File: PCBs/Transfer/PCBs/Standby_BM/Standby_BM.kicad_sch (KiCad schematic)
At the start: 30 parts, among them J1 SARI, J10 BL OUT, J11 5V IN, J12 LCD OUT 5V, J16 Address Select 0, J17 Address Select 1, J18 VVI PWR, J19 STBY AIR, J2 LOWER PWR, J20 AIR STPR, J21 AIR PWR, J3 UPPER PWR, J4 RWR BRT (ANALOG), J5 OLED PWR SEL, J6 STANDBY ALT, J7 STBY VVI, J8 VVI STPR, J9 BL IN, P1 Power, P2 Analog, P3 Analog, P4 Digital, P5 PWM, P6 PWM, P7 Communication

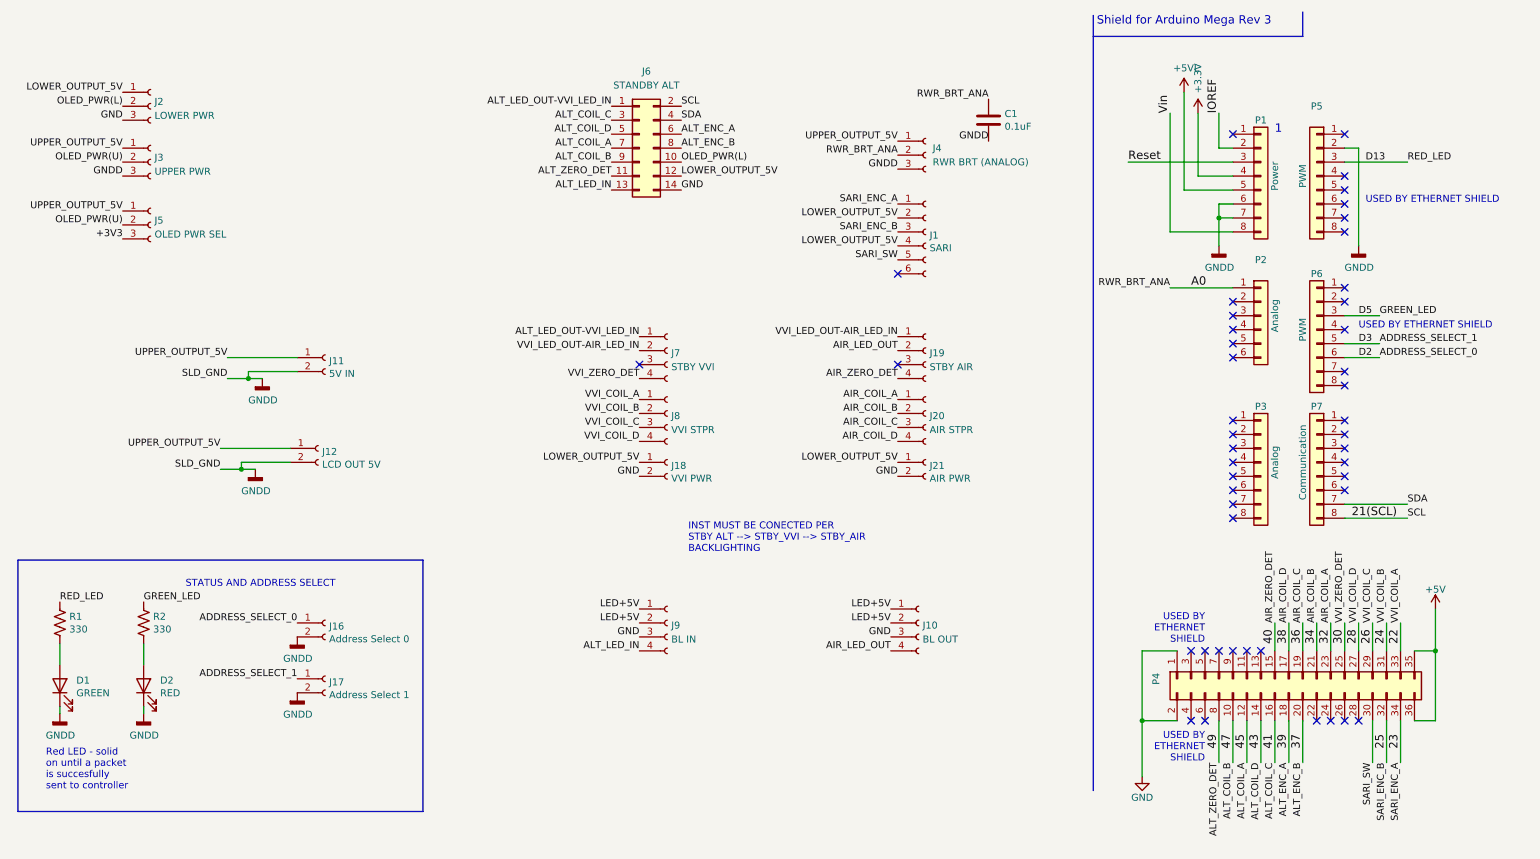
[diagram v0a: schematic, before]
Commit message: Ben4
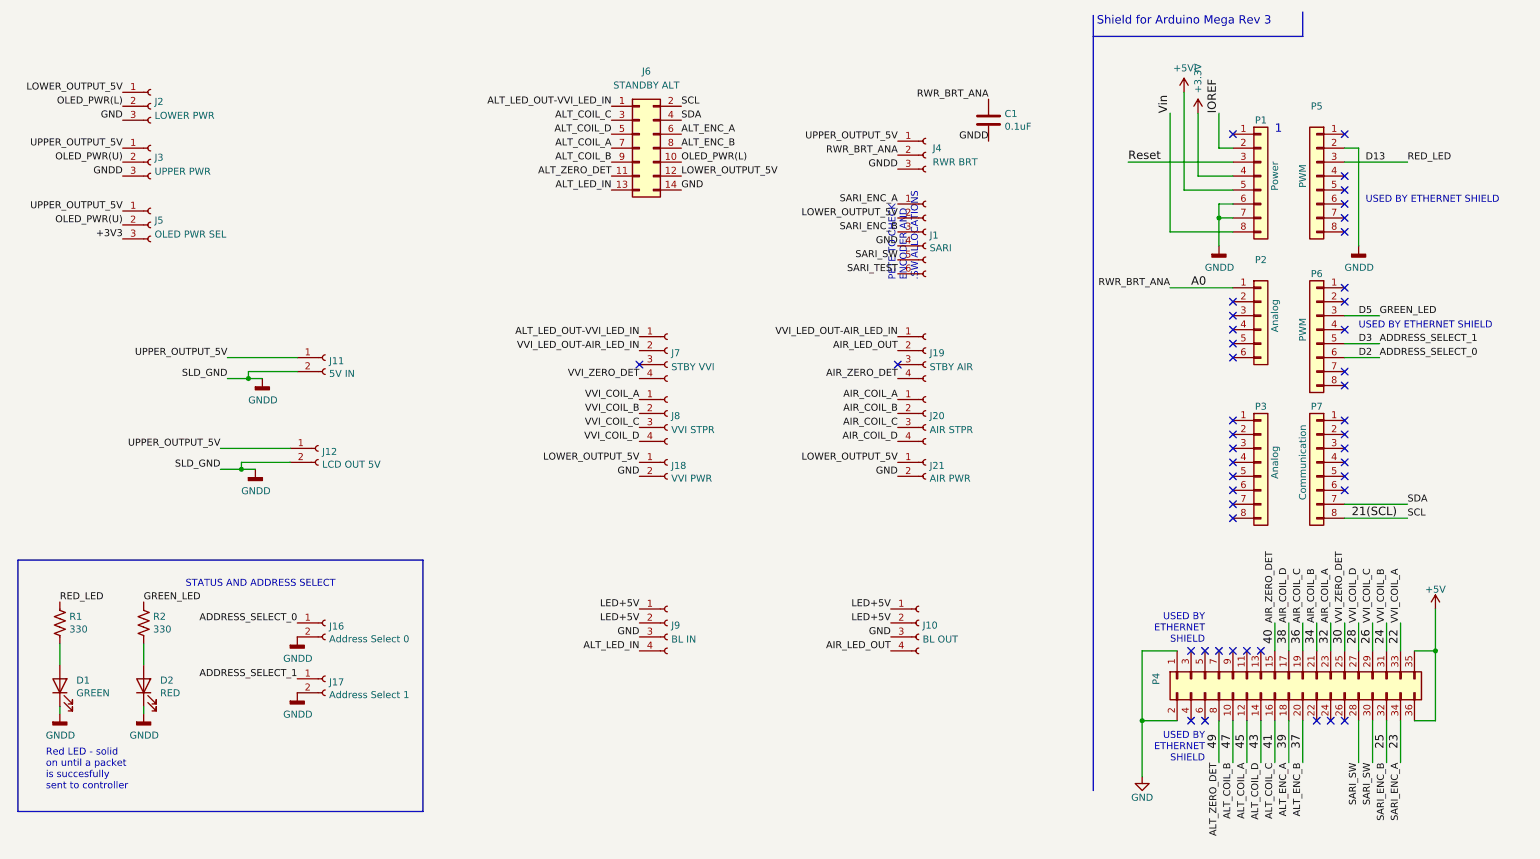
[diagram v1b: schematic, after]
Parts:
- J18, J21: footprint Connector_Molex:Molex_KK-254_AE-6410-06A_1x02_P2.54mm_Vertical -> Connector_Molex:Molex_KK-254_AE-6410-02A_1x02_P2.54mm_Vertical
- J2, J3: footprint Connector_Molex:Molex_KK-254_AE-6410-06A_1x03_P2.54mm_Vertical -> Connector_Molex:Molex_KK-254_AE-6410-03A_1x03_P2.54mm_Vertical
- J20, J7, J8: footprint Connector_Molex:Molex_KK-254_AE-6410-06A_1x04_P2.54mm_Vertical -> Connector_Molex:Molex_KK-254_AE-6410-04A_1x04_P2.54mm_Vertical
- J4: value RWR BRT (ANALOG) -> RWR BRT; footprint Connector_Molex:Molex_KK-254_AE-6410-06A_1x03_P2.54mm_Vertical -> Connector_Molex:Molex_KK-254_AE-6410-03A_1x03_P2.54mm_Vertical
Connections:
- net GND: now also J1.4 (Pin_4)
- net LOWER_OUTPUT_5V: no longer J1.4 (Pin_4)
- net SARI_SW: now also P4.28 (Pin_28)
- net SARI_TEST: now reaches J1.6 (Pin_6)
- no-connect marks 46 -> 44
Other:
- note added: "PETE TO CHECK ENCODER AND .SW ALLOCATIONS"
- note removed: "INST MUST BE CONECTED PER STBY ALT --> STBY_VVI --> STBY_AIR BACKLIGHTING"
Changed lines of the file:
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@@
   (no_connect (at 234.95 128.27))
   (no_connect (at 257.81 49.53))
-  (no_connect (at 176.53 59.69))
   (no_connect (at 242.57 128.27))
   (no_connect (at 257.81 41.91))
@@
   (no_connect (at 257.81 80.01))
   (no_connect (at 257.81 93.98))
-  (no_connect (at 260.35 140.97))
   (no_connect (at 237.49 67.31))
   (no_connect (at 257.81 88.9))
@@
     (stroke (width 0) (type default) (color 0 0 0 0))
   )
+  (wire (pts (xy 260.35 140.97) (xy 260.35 148.59))
+    (stroke (width 0) (type default) (color 0 0 0 0))
+  )
   (wire (pts (xy 54.61 74.93) (xy 67.31 74.93))
     (stroke (width 0) (type default) (color 0 0 0 0))
@@
     (effects (font (size 1.524 1.524)) (justify left bottom))
   )
-  (text "INST MUST BE CONECTED PER\nSTBY ALT --> STBY_VVI --> STBY_AIR\nBACKLIGHTING"
-    (at 138.43 110.49 0)
+  (text "PETE TO CHECK \nENCODER AND \n.SW ALLOCATIONS" (at 180.34 60.96 90)
     (effects (font (size 1.27 1.27)) (justify left bottom))
   )
@@
     (effects (font (size 1.27 1.27)) (justify right bottom))
   )
+  (label "SARI_SW" (at 260.35 148.59 270)
+    (effects (font (size 1.27 1.27)) (justify right bottom))
+  )
   (label "UPPER_OUTPUT_5V" (at 35.56 48.26 180)
     (effects (font (size 1.27 1.27)) (justify right bottom))
@@
     (effects (font (size 1.27 1.27)) (justify right bottom))
   )
+  (label "SARI_TEST" (at 176.53 59.69 180)
+    (effects (font (size 1.27 1.27)) (justify right bottom))
+  )
   (label "VVI_COIL_C" (at 262.89 123.19 90)
     (effects (font (size 1.27 1.27)) (justify left bottom))
   )
-  (label "LOWER_OUTPUT_5V" (at 176.53 54.61 180)
+  (label "GND" (at 176.53 54.61 180)
     (effects (font (size 1.27 1.27)) (justify right bottom))
   )
@@
       (effects (font (size 1.27 1.27)) (justify left))
     )
-    (property "Footprint" "Connector_Molex:Molex_KK-254_AE-6410-06A_1x02_P2.54mm_Vertical" (id 2) (at 181.61 93.98 0)
+    (property "Footprint" "Connector_Molex:Molex_KK-254_AE-6410-02A_1x02_P2.54mm_Vertical" (id 2) (at 181.61 93.98 0)
       (effects (font (size 1.27 1.27)) hide)
     )
@@
       (effects (font (size 1.27 1.27)) (justify left))
     )
-    (property "Footprint" "Connector_Molex:Molex_KK-254_AE-6410-06A_1x03_P2.54mm_Vertical" (id 2) (at 40.64 39.37 0)
+    (property "Footprint" "Connector_Molex:Molex_KK-254_AE-6410-03A_1x03_P2.54mm_Vertical" (id 2) (at 40.64 39.37 0)
       (effects (font (size 1.27 1.27)) hide)
     )
@@
       (effects (font (size 1.27 1.27)) (justify left))
     )
-    (property "Value" "RWR BRT (ANALOG)" (id 1) (at 182.88 39.3699 0)
-      (effects (font (size 1.27 1.27)) (justify left))
-    )
-    (property "Footprint" "Connector_Molex:Molex_KK-254_AE-6410-06A_1x03_P2.54mm_Vertical" (id 2) (at 181.61 38.1 0)
+    (property "Value" "RWR BRT" (id 1) (at 182.88 39.3699 0)
+      (effects (font (size 1.27 1.27)) (justify left))
+    )
+    (property "Footprint" "Connector_Molex:Molex_KK-254_AE-6410-03A_1x03_P2.54mm_Vertical" (id 2) (at 181.61 38.1 0)
       (effects (font (size 1.27 1.27)) hide)
     )
@@
       (effects (font (size 1.27 1.27)) (justify left))
     )
-    (property "Footprint" "Connector_Molex:Molex_KK-254_AE-6410-06A_1x04_P2.54mm_Vertical" (id 2) (at 134.62 85.09 0)
+    (property "Footprint" "Connector_Molex:Molex_KK-254_AE-6410-04A_1x04_P2.54mm_Vertical" (id 2) (at 134.62 85.09 0)
       (effects (font (size 1.27 1.27)) hide)
     )
@@
       (effects (font (size 1.27 1.27)) (justify left))
     )
-    (property "Footprint" "Connector_Molex:Molex_KK-254_AE-6410-06A_1x02_P2.54mm_Vertical" (id 2) (at 134.62 93.98 0)
+    (property "Footprint" "Connector_Molex:Molex_KK-254_AE-6410-02A_1x02_P2.54mm_Vertical" (id 2) (at 134.62 93.98 0)
       (effects (font (size 1.27 1.27)) hide)
     )
@@
       (effects (font (size 1.27 1.27)) (justify left))
     )
-    (property "Footprint" "Connector_Molex:Molex_KK-254_AE-6410-06A_1x04_P2.54mm_Vertical" (id 2) (at 181.61 85.09 0)
+    (property "Footprint" "Connector_Molex:Molex_KK-254_AE-6410-04A_1x04_P2.54mm_Vertical" (id 2) (at 181.61 85.09 0)
       (effects (font (size 1.27 1.27)) hide)
     )
@@
       (effects (font (size 1.27 1.27)) (justify left))
     )
-    (property "Footprint" "Connector_Molex:Molex_KK-254_AE-6410-06A_1x03_P2.54mm_Vertical" (id 2) (at 40.64 29.21 0)
+    (property "Footprint" "Connector_Molex:Molex_KK-254_AE-6410-03A_1x03_P2.54mm_Vertical" (id 2) (at 40.64 29.21 0)
       (effects (font (size 1.27 1.27)) hide)
     )
@@
       (effects (font (size 1.27 1.27)) (justify left))
     )
-    (property "Footprint" "Connector_Molex:Molex_KK-254_AE-6410-06A_1x04_P2.54mm_Vertical" (id 2) (at 134.62 73.66 0)
+    (property "Footprint" "Connector_Molex:Molex_KK-254_AE-6410-04A_1x04_P2.54mm_Vertical" (id 2) (at 134.62 73.66 0)
       (effects (font (size 1.27 1.27)) hide)
     )
@@
     )
     (path "/c22b76af-83c5-4afc-966d-2b2522fe5468"
-      (reference "J2") (unit 1) (value "LOWER PWR") (footprint "Connector_Molex:Molex_KK-254_AE-6410-06A_1x03_P2.54mm_Vertical")
+      (reference "J2") (unit 1) (value "LOWER PWR") (footprint "Connector_Molex:Molex_KK-254_AE-6410-03A_1x03_P2.54mm_Vertical")
     )
     (path "/65a4c4e4-5453-4bf7-a172-864899e675ae"
-      (reference "J3") (unit 1) (value "UPPER PWR") (footprint "Connector_Molex:Molex_KK-254_AE-6410-06A_1x03_P2.54mm_Vertical")
+      (reference "J3") (unit 1) (value "UPPER PWR") (footprint "Connector_Molex:Molex_KK-254_AE-6410-03A_1x03_P2.54mm_Vertical")
     )
     (path "/73cc9871-345e-4600-8dae-99243954c002"
-      (reference "J4") (unit 1) (value "RWR BRT (ANALOG)") (footprint "Connector_Molex:Molex_KK-254_AE-6410-06A_1x03_P2.54mm_Vertical")
+      (reference "J4") (unit 1) (value "RWR BRT") (footprint "Connector_Molex:Molex_KK-254_AE-6410-03A_1x03_P2.54mm_Vertical")
     )
     (path "/957ca4f0-bf1c-4c34-9635-0d51deb78cc9"
@@
     )
     (path "/fb357ca4-117b-4eb9-840e-613d17fa264a"
-      (reference "J7") (unit 1) (value "STBY VVI") (footprint "Connector_Molex:Molex_KK-254_AE-6410-06A_1x04_P2.54mm_Vertical")
+      (reference "J7") (unit 1) (value "STBY VVI") (footprint "Connector_Molex:Molex_KK-254_AE-6410-04A_1x04_P2.54mm_Vertical")
     )
     (path "/8f732ad9-d721-48aa-9c73-5b2fe4f8060e"
-      (reference "J8") (unit 1) (value "VVI STPR") (footprint "Connector_Molex:Molex_KK-254_AE-6410-06A_1x04_P2.54mm_Vertical")
+      (reference "J8") (unit 1) (value "VVI STPR") (footprint "Connector_Molex:Molex_KK-254_AE-6410-04A_1x04_P2.54mm_Vertical")
     )
     (path "/2b5af193-10ae-4588-b4bc-7cafb0ecf247"
@@
     )
     (path "/9a177cfc-2d30-4bcd-b935-19e3ad767135"
-      (reference "J18") (unit 1) (value "VVI PWR") (footprint "Connector_Molex:Molex_KK-254_AE-6410-06A_1x02_P2.54mm_Vertical")
+      (reference "J18") (unit 1) (value "VVI PWR") (footprint "Connector_Molex:Molex_KK-254_AE-6410-02A_1x02_P2.54mm_Vertical")
     )
     (path "/f221fa5d-17fb-49a3-83d7-c6c946abfdb8"
@@
     )
     (path "/a7c831fd-41d8-4930-b242-8b9ab0569617"
-      (reference "J20") (unit 1) (value "AIR STPR") (footprint "Connector_Molex:Molex_KK-254_AE-6410-06A_1x04_P2.54mm_Vertical")
+      (reference "J20") (unit 1) (value "AIR STPR") (footprint "Connector_Molex:Molex_KK-254_AE-6410-04A_1x04_P2.54mm_Vertical")
     )
     (path "/26cd68bf-ccf7-4c3a-960d-1e8cb7e6aef1"
-      (reference "J21") (unit 1) (value "AIR PWR") (footprint "Connector_Molex:Molex_KK-254_AE-6410-06A_1x02_P2.54mm_Vertical")
+      (reference "J21") (unit 1) (value "AIR PWR") (footprint "Connector_Molex:Molex_KK-254_AE-6410-02A_1x02_P2.54mm_Vertical")
     )
     (path "/00000000-0000-0000-0000-000056d71773"

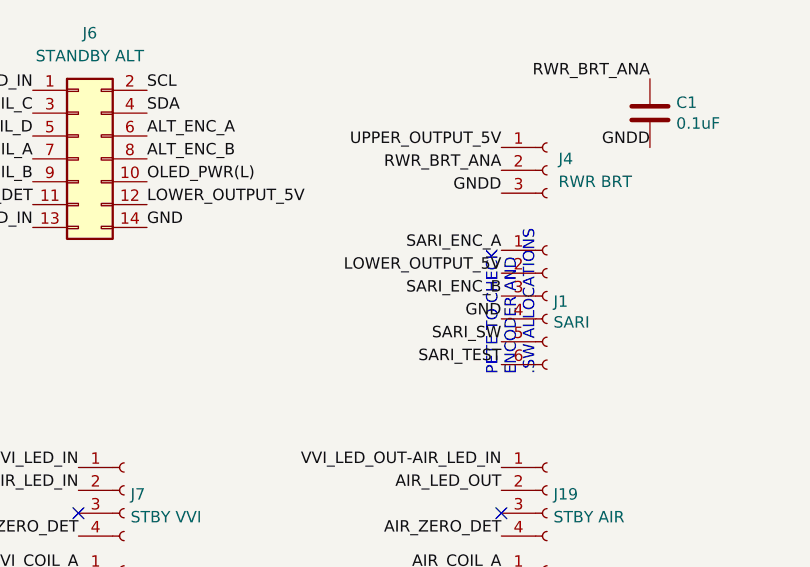
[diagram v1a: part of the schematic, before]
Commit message: Standy BM Good
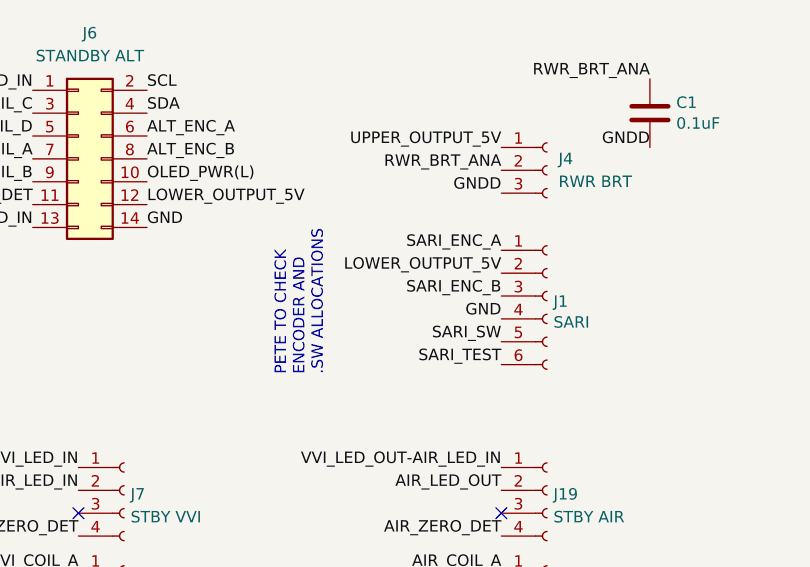
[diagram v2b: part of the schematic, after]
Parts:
- J6: footprint Connector_PinHeader_2.54mm:PinHeader_2x07_P2.54mm_Vertical -> Connector_IDC:IDC-Header_2x07_P2.54mm_Vertical
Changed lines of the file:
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@@
     (effects (font (size 1.524 1.524)) (justify left bottom))
   )
-  (text "PETE TO CHECK \nENCODER AND \n.SW ALLOCATIONS" (at 180.34 60.96 90)
+  (text "PETE TO CHECK \nENCODER AND \n.SW ALLOCATIONS" (at 156.845 60.96 90)
     (effects (font (size 1.27 1.27)) (justify left bottom))
   )
@@
     (property "Reference" "J6" (id 0) (at 130.81 22.86 0))
     (property "Value" "STANDBY ALT" (id 1) (at 130.81 25.4 0))
-    (property "Footprint" "Connector_PinHeader_2.54mm:PinHeader_2x07_P2.54mm_Vertical" (id 2) (at 129.54 36.83 0)
+    (property "Footprint" "Connector_IDC:IDC-Header_2x07_P2.54mm_Vertical" (id 2) (at 129.54 36.83 0)
       (effects (font (size 1.27 1.27)) hide)
     )
@@
     )
     (path "/d4fed0f0-0ead-4947-834c-d0aad2598f56"
-      (reference "J6") (unit 1) (value "STANDBY ALT") (footprint "Connector_PinHeader_2.54mm:PinHeader_2x07_P2.54mm_Vertical")
+      (reference "J6") (unit 1) (value "STANDBY ALT") (footprint "Connector_IDC:IDC-Header_2x07_P2.54mm_Vertical")
     )
     (path "/fb357ca4-117b-4eb9-840e-613d17fa264a"
